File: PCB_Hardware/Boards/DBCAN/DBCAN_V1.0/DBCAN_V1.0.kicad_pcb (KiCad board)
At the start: 4 copper layers, 47 x 30 mm, 58 parts, among them J1 Conn_ARM_SWD_TagConnect_TC203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, J11 GT-USB-7010ASV, J2 SM04B-PASS-TBT, J3 SM04B-PASS-TBT, Q1 SI2302, Q2 SI2302, Q3 SI2302, Q4 SI2302, U1 STM32G0B1KBT6TR, U10 TPD2E2U06DCK, U16 CAT24C256, U2 TCAN1048AVDMTRQ1, U3 MCP1802T-3302I/OT, Y1 ASEMB-8.000MHZ-XY-T

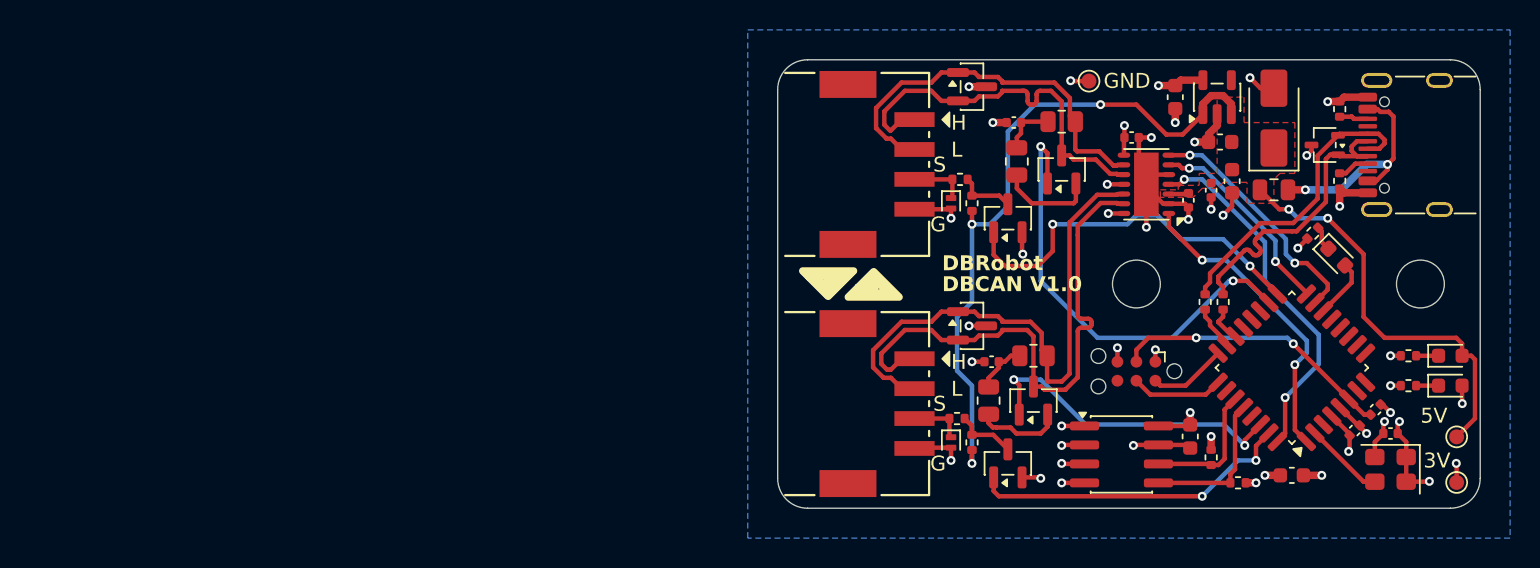
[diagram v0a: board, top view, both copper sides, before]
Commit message: First version of DBCAN board
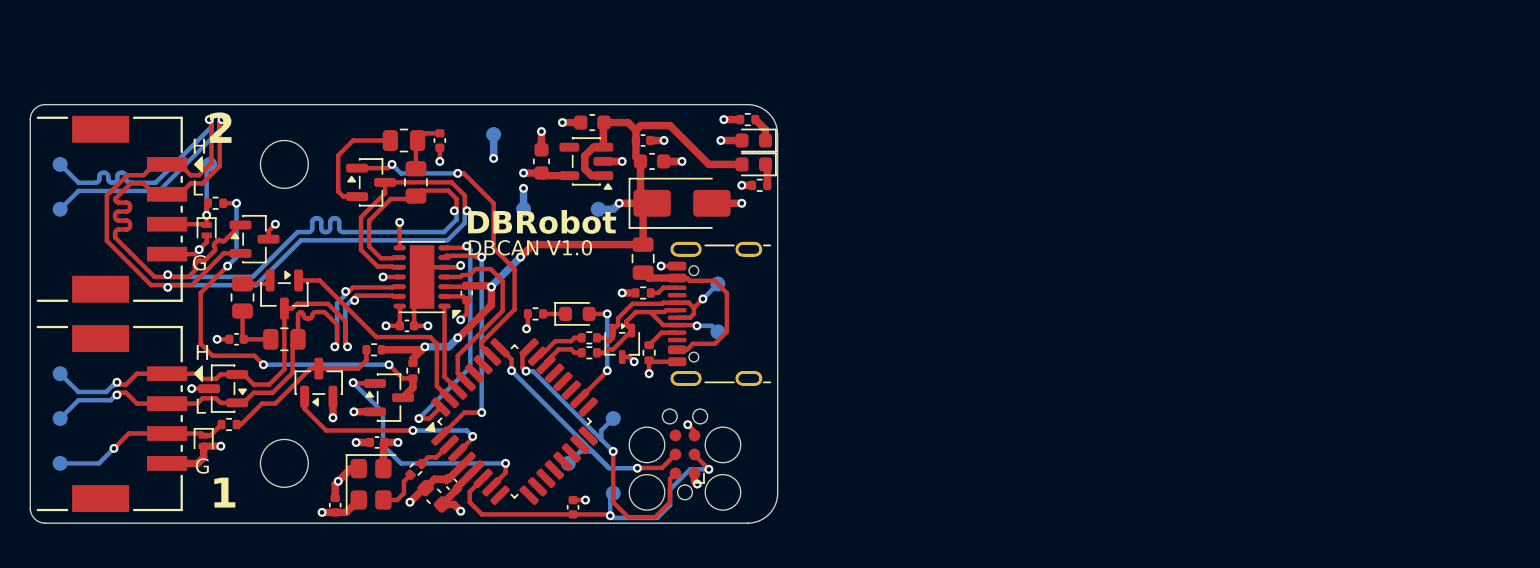
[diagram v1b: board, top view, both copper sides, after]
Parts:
- removed C37: 4.7u, Capacitor_SMD:C_0603_1608Metric
- removed C38, C6, C7: 100n, Capacitor_SMD:C_0402_1005Metric
- removed C39, C40: 1u, Capacitor_SMD:C_0603_1608Metric
- removed C46: 100n, Capacitor_SMD:C_0603_1608Metric
- removed C8: 10n, Capacitor_SMD:C_0402_1005Metric
- removed D10: SMAJ5.0A, Diode_SMD:D_SMA
- removed J11: GT-USB-7010ASV, Connector_USB:USB_C_Receptacle_G-Switch_GT-USB-7010ASV
- removed R1, R2: 60, Resistor_SMD:R_0805_2012Metric
- removed R27, R28: 4.7k, Resistor_SMD:R_0402_1005Metric
- removed R47, R48: 5.1k, Resistor_SMD:R_0402_1005Metric
- removed R49, R50, R53: 2.2k, Resistor_SMD:R_0402_1005Metric
- removed R51, R52: 22, Resistor_SMD:R_0402_1005Metric
- removed U10: TPD2E2U06DCK, Package_TO_SOT_SMD:SOT-323_SC-70
- removed U16: CAT24C256, Package_SO:SOIC-8_3.9x4.9mm_P1.27mm
- added C11: 4.7u, Capacitor_SMD:C_0603_1608Metric, F.Cu at (131.6, 79.8)
- added C12: 100n, Capacitor_SMD:C_0402_1005Metric, F.Cu at (131.0, 78.4)
- added C13: 1u, Capacitor_SMD:C_0603_1608Metric, F.Cu at (127.6, 77.2)
- added C14: 1u, Capacitor_SMD:C_0603_1608Metric, F.Cu at (124.2, 79.8)
- added C15: 100n, Capacitor_SMD:C_0402_1005Metric, F.Cu at (119.2, 88.6)
- added C16: 100n, Capacitor_SMD:C_0402_1005Metric, F.Cu at (115.2, 90.8)
- added C17: 4.7n, Capacitor_SMD:C_0402_1005Metric, F.Cu at (103.8, 91.7)
- added C18: 4.7n, Capacitor_SMD:C_0402_1005Metric, F.Cu at (117.4, 78.4)
- added D8: BLUE, LED_SMD:LED_0603_1608Metric, F.Cu at (126.6, 90.0)
- added J4: SM04B-PASS-TBT, DBRobot:CONN_JST_SM04B-PASS, F.Cu at (95.0, 83.0)
- added R10: 60.4, Resistor_SMD:R_0805_2012Metric, F.Cu at (104.2, 88.9)
- added R11: 60.4, Resistor_SMD:R_0805_2012Metric, F.Cu at (115.8, 81.2)
- added R12: 60.4, Resistor_SMD:R_0805_2012Metric, F.Cu at (115.0, 78.4)
- added R13: 10k, Resistor_SMD:R_0402_1005Metric, F.Cu at (113.0, 92.4)
- added R14: 10k, Resistor_SMD:R_0402_1005Metric, F.Cu at (115.6, 93.8)
- added R15: 1k, Resistor_SMD:R_0402_1005Metric, F.Cu at (103.3, 97.4)
- added R16: 1k, Resistor_SMD:R_0402_1005Metric, F.Cu at (102.4, 82.6)
- added R17: 2.2k, Resistor_SMD:R_0402_1005Metric, F.Cu at (123.8, 90.0)
- added R18: 0, Resistor_SMD:R_0402_1005Metric, F.Cu at (115.8, 100.4)
- added R9: 60.4, Resistor_SMD:R_0805_2012Metric, F.Cu at (107.0, 91.7)
- added TP10: TestPoint, TestPoint:TestPoint_Pad_D1.0mm, B.Cu at (92.0, 83.0)
- added TP11: TestPoint, TestPoint:TestPoint_Pad_D1.0mm, B.Cu at (102.0, 80.0)
- added TP12: TestPoint, TestPoint:TestPoint_Pad_D1.0mm, B.Cu at (136.0, 91.2)
- added TP13: TestPoint, TestPoint:TestPoint_Pad_D1.0mm, B.Cu at (136.0, 88.0)
- added TP14: TestPoint, TestPoint:TestPoint_Pad_D1.0mm, B.Cu at (129.0, 102.0)
- added TP4: TestPoint, TestPoint:TestPoint_Pad_D1.0mm, B.Cu at (126.0, 100.0)
- added TP5: TestPoint, TestPoint:TestPoint_Pad_D1.0mm, B.Cu at (129.0, 97.0)
- added TP6: TestPoint, TestPoint:TestPoint_Pad_D1.0mm, B.Cu at (92.0, 94.0)
- added TP7: TestPoint, TestPoint:TestPoint_Pad_D1.0mm, B.Cu at (92.0, 97.0)
- added TP8: TestPoint, TestPoint:TestPoint_Pad_D1.0mm, B.Cu at (92.0, 100.0)
- added TP9: TestPoint, TestPoint:TestPoint_Pad_D1.0mm, B.Cu at (92.0, 80.0)
- added U4: TCAN1048AVDMTRQ1, Package_DFN_QFN:DFN-14-1EP_3x4.5mm_P0.65mm_EP1.65x4.25mm, F.Cu at (116.2, 87.5)
- C4, C5: value 4.7n -> 100n
- D2: value PESD1CAN -> SMAJ5.0A; footprint Package_TO_SOT_SMD:SOT-23 -> Diode_SMD:D_SMA
- D3: value PESD1CAN -> RED; footprint Package_TO_SOT_SMD:SOT-23 -> LED_SMD:LED_0603_1608Metric
- D4: value RED -> PESD5V0L1UL; footprint LED_SMD:LED_0603_1608Metric -> Diode_SMD:D_SOD-882
- D5, D6: value PESD5V0L1UL -> PESD1CAN; footprint Diode_SMD:D_SOD-882 -> Package_TO_SOT_SMD:SOT-23
- D7: value BLUE -> PESD5V0L1UL; footprint LED_SMD:LED_0603_1608Metric -> Diode_SMD:D_SOD-882
- F1: value MF-PSMF050X-2 -> BSMD0805-050-24V
- J1: value Conn_ARM_SWD_TagConnect_TC2030-NL -> Conn_ARM_SWD_TagConnect_TC2030; footprint Connector:Tag-Connect_TC2030-IDC-NL_2x03_P1.27mm_Vertical -> Connector:Tag-Connect_TC2030-IDC-FP_2x03_P1.27mm_Vertical
- J2: value SM04B-PASS-TBT -> GT-USB-7010ASV; footprint DBRobot:CONN_JST_SM04B-PASS -> Connector_USB:USB_C_Receptacle_G-Switch_GT-USB-7010ASV
- R3, R4: value 60 -> 2.2k; footprint Resistor_SMD:R_0805_2012Metric -> Resistor_SMD:R_0402_1005Metric
- R5, R6: value 10k -> 5.1k
- R7, R8: value 100k -> 0
- TP1, TP2, TP3: moved to B.Cu
- U1: value STM32G0B1KBT6TR -> STM32G0B1KBT6
- U2: value TCAN1048AVDMTRQ1 -> MCP1802T-3302I/OT; footprint Package_DFN_QFN:DFN-14-1EP_3x4.5mm_P0.65mm_EP1.65x4.25mm -> Package_TO_SOT_SMD:SOT-23-5
- U3: value MCP1802T-3302I/OT -> TPD2E2U06DCK; footprint Package_TO_SOT_SMD:SOT-23-5 -> Package_TO_SOT_SMD:SOT-323_SC-70
- Y1: value ASEMB-8.000MHZ-XY-T -> ASEM1-24.000MHZ-LC-T
- moved D4 83.5 mm to (101.6, 98.5), turned to -90 degrees
- moved H2 76.4 mm to (107.0, 80.0)
- moved D7 75.6 mm to (101.8, 84.4), turned to -90 degrees
- moved Y1 68.2 mm to (112.8, 101.4), turned to -90 degrees
- moved TP1 64.3 mm to (123.0, 83.0), turned to 180 degrees
- moved C3 60.6 mm to (110.4, 102.8)
- moved C2 60.5 mm to (118.2, 101.4), turned to -45 degrees
- moved TP2 60.3 mm to (128.0, 83.0), turned to 180 degrees
- moved H1 58.2 mm to (107.0, 100.0)
- moved C1 57.4 mm to (117.0, 102.2), turned to -45 degrees
- moved J3 52.8 mm to (95.0, 97.0)
- moved U1 52.1 mm to (122.4, 97.2), turned to 45 degrees
- moved Q1 50.6 mm to (107.0, 88.7), turned to -90 degrees
- moved D5 50.3 mm to (102.9, 95.0), turned to 180 degrees
- moved D1 48.8 mm to (138.4, 78.4), turned to 180 degrees
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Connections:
- C3 pad 1: +5V -> +3.3V
- C4 pad 1: Net-(C4-Pad1) -> +3.3V
- C5 pad 1: Net-(C5-Pad1) -> GND
- C5 pad 2: GND -> /MCU/NRST
- D1 pad 2: +5V -> +3.3V
- D2 pad 1: /CANFD/CANFD1- -> +5V
- D2 pad 2: /CANFD/CANFD1+ -> GND
- D3 pad 1: /CANFD/CANFD2- -> Net-(D3-K)
- D3 pad 2: /CANFD/CANFD2+ -> +5V
- D4 pad 1: Net-(D4-K) -> /CANFD/SEQ1_PIN
- D4 pad 2: +3.3V -> GND
- D5 pad 1: Net-(D5-K) -> /CANFD/CANFD1-
- D5 pad 2: GND -> /CANFD/CANFD1+
- D6 pad 1: Net-(D6-K) -> /CANFD/CANFD2-
- D6 pad 2: GND -> /CANFD/CANFD2+
- D7 pad 1: Net-(D7-K) -> /CANFD/SEQ2_PIN
- D7 pad 2: Net-(D7-A) -> GND
- J3 pad 1: /CANFD/CANFD2+ -> /CANFD/CANFD1+
- J3 pad 2: /CANFD/CANFD2- -> /CANFD/CANFD1-
- J3 pad 3: Net-(D5-K) -> /CANFD/SEQ1_PIN
- R3 pad 1: /CANFD/CANFD2- -> GND
- R3 pad 2: Net-(C5-Pad1) -> Net-(D1-K)
- R4 pad 1: Net-(C5-Pad1) -> GND
- R4 pad 2: Net-(Q2-S) -> Net-(D3-K)
- R5 pad 1: Net-(Q3-D) -> Net-(J2-CC1)
- R5 pad 2: +5V -> GND
- R6 pad 1: Net-(Q4-D) -> Net-(J2-CC2)
- R6 pad 2: +5V -> GND
- R7 pad 1: Net-(D6-K) -> /MCU/USB_D-
- R7 pad 2: Net-(Q3-D) -> /USB/D-
- R8 pad 1: Net-(D5-K) -> /MCU/USB_D+
- R8 pad 2: Net-(Q4-D) -> /USB/D+
- TP1 pad 1: +5V -> +3.3V
- TP2 pad 1: +3.3V -> +5V
- U1 pad 1: /CANFD/CANFD_TX1 -> /CANFD/CANFD_TX2
- U1 pad 14: Net-(D7-A) -> unconnected-(U1-PA7-Pad14)
- U1 pad 15: /CANFD/CANFD_RX2 -> unconnected-(U1-PB0-Pad15)
- U1 pad 16: /CANFD/CANFD_TX2 -> unconnected-(U1-PB1-Pad16)
- U1 pad 17: /CANFD/SEQ2 -> unconnected-(U1-PB2-Pad17)
- U1 pad 18: /CANFD/TERM_R2 -> Net-(D8-A)
- U1 pad 26: unconnected-(U1-PA15-Pad26) -> /CANFD/TERM_R2
- U1 pad 27: /EEPROM/EEPROM_SCL -> unconnected-(U1-PB3-Pad27)
- U1 pad 28: /EEPROM/EEPROM_SDA -> unconnected-(U1-PB4-Pad28)
- U1 pad 29: unconnected-(U1-PB5-Pad29) -> /CANFD/CANFD_RX1
- U1 pad 3: unconnected-(U1-PC15-Pad3) -> /CANFD/SEQ1
- U1 pad 30: /CANFD/TERM_R1 -> /CANFD/CANFD_TX1
- U1 pad 31: /CANFD/SEQ1 -> /CANFD/TERM_R1
- U1 pad 32: /CANFD/CANFD_RX1 -> /CANFD/CANFD_RX2
- U1 pad 7: unconnected-(U1-PA0-Pad7) -> /CANFD/SEQ2
- U2 pad 1: /CANFD/CANFD_TX1 -> +5V
- U2 pad 4: /CANFD/CANFD_RX1 -> unconnected-(U2-NC-Pad4)
- U2 pad 5: GND -> +3.3V
- U3 pad 1: +5V -> /USB/D-
- U3 pad 2: GND -> /USB/D+
- U3 pad 3: +5V -> GND
- Y1 pad 3: Net-(U1-PC14) -> Net-(Y1-OUT)
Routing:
- net /CANFD/CANFD2-: track 26.5 -> 79.1 mm, vias 0 -> 3
- net /CANFD/CANFD2+: track 26.4 -> 77.7 mm, vias 0 -> 3
- net Net-(Q4-D): track 3.85 -> 28.0 mm, vias 0 -> 4
- net +5V: track 74.5 -> 54.0 mm
- net /MCU/SWDIO: track 5.23 -> 21.7 mm, vias 0 -> 2
- net /CANFD/CANFD_TX1: track 20.7 -> 5.98 mm, vias 2 -> 0
- net /MCU/SWCLK: track 6.20 -> 19.3 mm, vias 0 -> 2
- net /CANFD/SEQ1_PIN: track 0.00 -> 12.0 mm, vias 0 -> 1
- net /CANFD/CANFD_RX1: track 24.3 -> 12.6 mm, vias 2 -> 0
- net /EEPROM/EEPROM_SDA: track 10.2 -> 0.00 mm
- net GND: track 63.4 -> 53.3 mm, vias 33 -> 30
- net /EEPROM/EEPROM_SCL: track 8.91 -> 0.00 mm
- net /CANFD/TERM_R2: track 30.7 -> 22.3 mm
- net /CANFD/SEQ2: track 25.5 -> 17.2 mm
- net /USB/D+: track 20.4 -> 12.3 mm, vias 0 -> 1
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- removed copper zone on F.Cu, net +5V
- removed copper zone on B.Cu, net GND
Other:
- board size 47 x 30 mm -> 50 x 28 mm
- board text added: "3.3V"
- board text added: "H1"
- board text added: "H2"
- board text added: "L1"
- board text added: "L2"
- board text added: "NRST"
- board text added: "SEQ1"
- board text added: "SEQ2"
- board text added: "SWCLK"
- board text added: "SWDIO"
- board text removed: "3V"
- board text removed: "S"
